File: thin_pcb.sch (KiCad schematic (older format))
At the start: 151 parts, among them J01 Conn_01x02, J02 Conn_01x02, J04 Conn_01x02, J06 Conn_01x02, J07 Conn_01x02, J08 Conn_01x02, J1 USB_B_Micro, J11 Conn_01x03, J12 Conn_01x03, J13 Conn_01x03, J14 Conn_01x03, J15 Conn_01x03, J16 Conn_01x03, J17 Conn_01x03, J18 Conn_01x03, J2 AudioJack4_Ground, J21 Conn_01x07, J22 Conn_01x07, J23 Conn_01x07, J24 Conn_01x07, J25 Conn_01x07, J26 Conn_01x07, J27 Conn_01x07, J28 Conn_01x07, J3 AudioJack4_Ground, J31 Conn_01x07, J32 Conn_01x07, J33 Conn_01x07, J34 Conn_01x07, J35 Conn_01x07, J36 Conn_01x07, J37 Conn_01x07, J38 Conn_01x07, J4 Conn_01x06, J41 Conn_01x04, J42 Conn_01x04, J43 Conn_01x04, J44 Conn_01x04, J45 Conn_01x04, J46 Conn_01x04, J47 Conn_01x04, J48 Conn_01x04, J5 Conn_01x06, J51 Conn_01x01, J52 Conn_01x01, J53 Conn_01x01, J54 Conn_01x01, J55 Conn_01x01, J56 Conn_01x01, J57 Conn_01x01, J58 Conn_01x01, J6 Conn_02x02, J7 Conn_01x02, SW11 SW_Push, SW12 SW_Push, SW13 SW_Push, SW14 SW_Push, SW15 SW_Push, SW21 SW_Push, SW22 SW_Push, SW23 SW_Push, SW24 SW_Push, SW25 SW_Push, SW252 SW_Push, SW31 SW_Push, SW32 SW_Push, SW33 SW_Push, SW34 SW_Push, SW35 SW_Push, SW41 SW_Push, SW42 SW_Push, SW422 SW_Push, SW43 SW_Push, SW44 SW_Push, SW45 SW_Push, SW452 SW_Push, SW51 SW_Push, SW52 SW_Push, SW522 SW_Push, SW53 SW_Push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

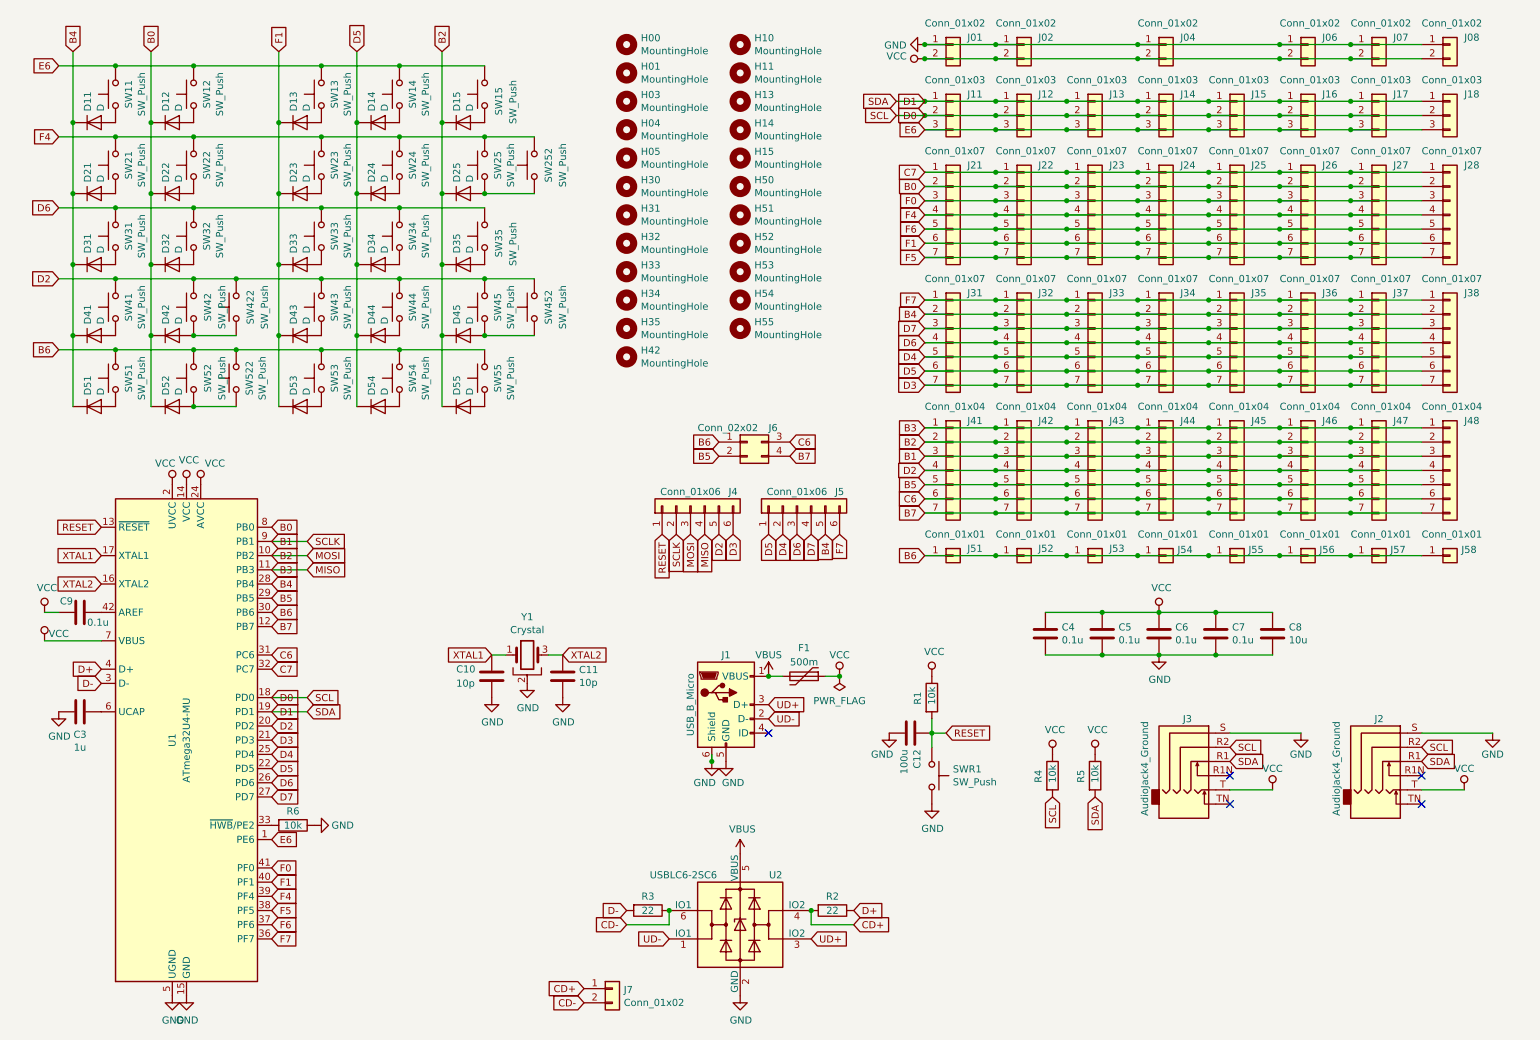
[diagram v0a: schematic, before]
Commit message: column pins
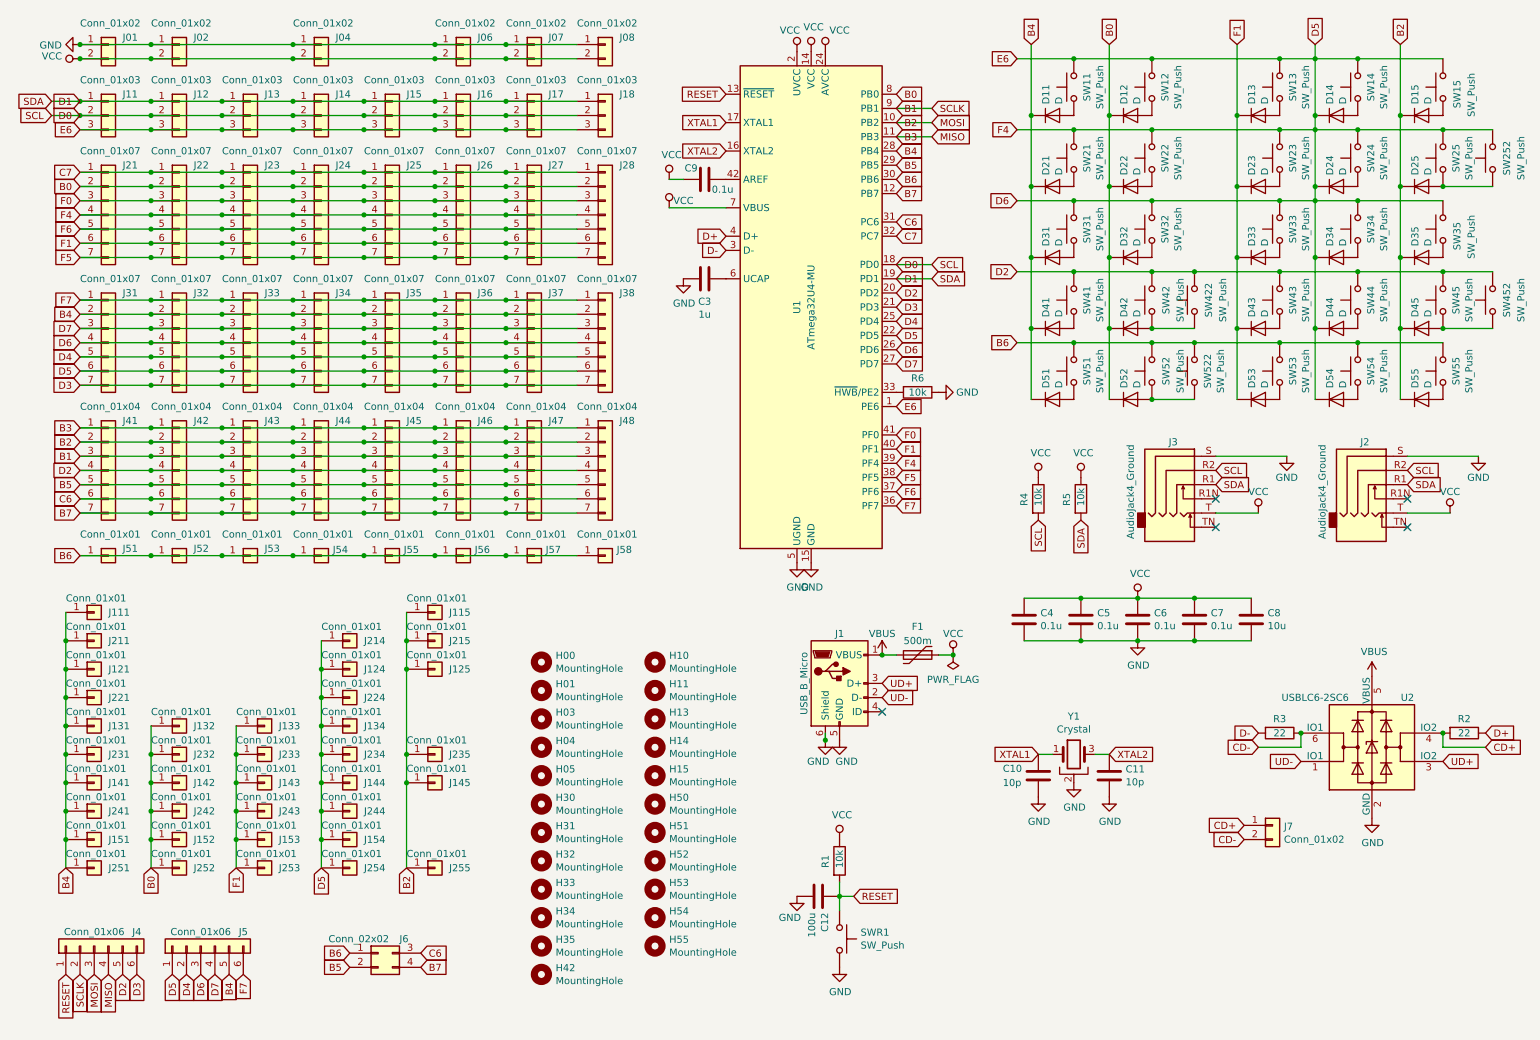
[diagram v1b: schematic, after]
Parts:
- added J111, J115, J121, J124, J125, J131, J132, J133, J134, J141, J142, J143, J144, J145, J151, J152, J153, J154, J211, J214, J215, J221, J224, J231, J232, J233, J234, J235, J241, J242, J243, J244, J251, J252, J253, J254, J255: Conn_01x01, lib:PinSocket_1x01_P2.54mm_Vertical, symbol Connector_Generic:Conn_01x01
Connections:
- net D6 is gone; now on net D5: J31.4 (Pin_4), J32.4 (Pin_4), J33.4 (Pin_4), J34.4 (Pin_4), J35.4 (Pin_4), J36.4 (Pin_4), J37.4 (Pin_4), J38.4 (Pin_4), J5.3 (Pin_3), SW31.2, SW32.2, SW33.2, SW34.2, SW35.2, U1.26 (PD6)
- net E6 is gone; now on net D5: J11.3 (Pin_3), J12.3 (Pin_3), J13.3 (Pin_3), J14.3 (Pin_3), J15.3 (Pin_3), J16.3 (Pin_3), J17.3 (Pin_3), J18.3 (Pin_3), SW11.2, SW12.2, SW13.2, SW14.2, SW15.2, U1.1 (PE6)
- net F4 is gone; now on net D5: J21.4 (Pin_4), J22.4 (Pin_4), J23.4 (Pin_4), J24.4 (Pin_4), J25.4 (Pin_4), J26.4 (Pin_4), J27.4 (Pin_4), J28.4 (Pin_4), SW21.2, SW22.2, SW23.2, SW24.2, SW25.2, SW252.2, U1.39 (PF4)
- net B0: now also J132.1 (Pin_1), J142.1 (Pin_1), J152.1 (Pin_1), J232.1 (Pin_1), J242.1 (Pin_1), J252.1 (Pin_1)
- net B2: now also J115.1 (Pin_1), J125.1 (Pin_1), J145.1 (Pin_1), J215.1 (Pin_1), J235.1 (Pin_1), J255.1 (Pin_1)
- net B4: now also J111.1 (Pin_1), J121.1 (Pin_1), J131.1 (Pin_1), J141.1 (Pin_1), J151.1 (Pin_1), J211.1 (Pin_1), J221.1 (Pin_1), J231.1 (Pin_1), J241.1 (Pin_1), J251.1 (Pin_1)
- net D5: now also J124.1 (Pin_1), J134.1 (Pin_1), J144.1 (Pin_1), J154.1 (Pin_1), J214.1 (Pin_1), J224.1 (Pin_1), J234.1 (Pin_1), J244.1 (Pin_1), J254.1 (Pin_1)
- net F1: now also J133.1 (Pin_1), J143.1 (Pin_1), J153.1 (Pin_1), J233.1 (Pin_1), J243.1 (Pin_1), J253.1 (Pin_1)
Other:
- moved on the sheet: C10, C11, C12, C3, C4, C5, C6, C7, C8, C9, D11, D12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
